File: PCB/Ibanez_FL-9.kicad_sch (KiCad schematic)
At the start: 156 parts, among them J1 INPUT, J2 OUTPUT, J3 EXT_DC, Q101 2SC2458GR, Q102 2SC2458GR, Q103 2SK44SPC, Q104 2SC2458GR, Q105 2SC2458GR, Q106 2SC2458GR, Q107 2SA1048Y/GR, Q108A1001 2SC1583F, Q108B1001 2SC1583F, Q109 2SC2458GR, SW1 NORMAL/EFFECT, U101 TL022, U102 TL022, U103 TL022, U104 MN3207, U105 MN3102, U106 LM78L05_TO92

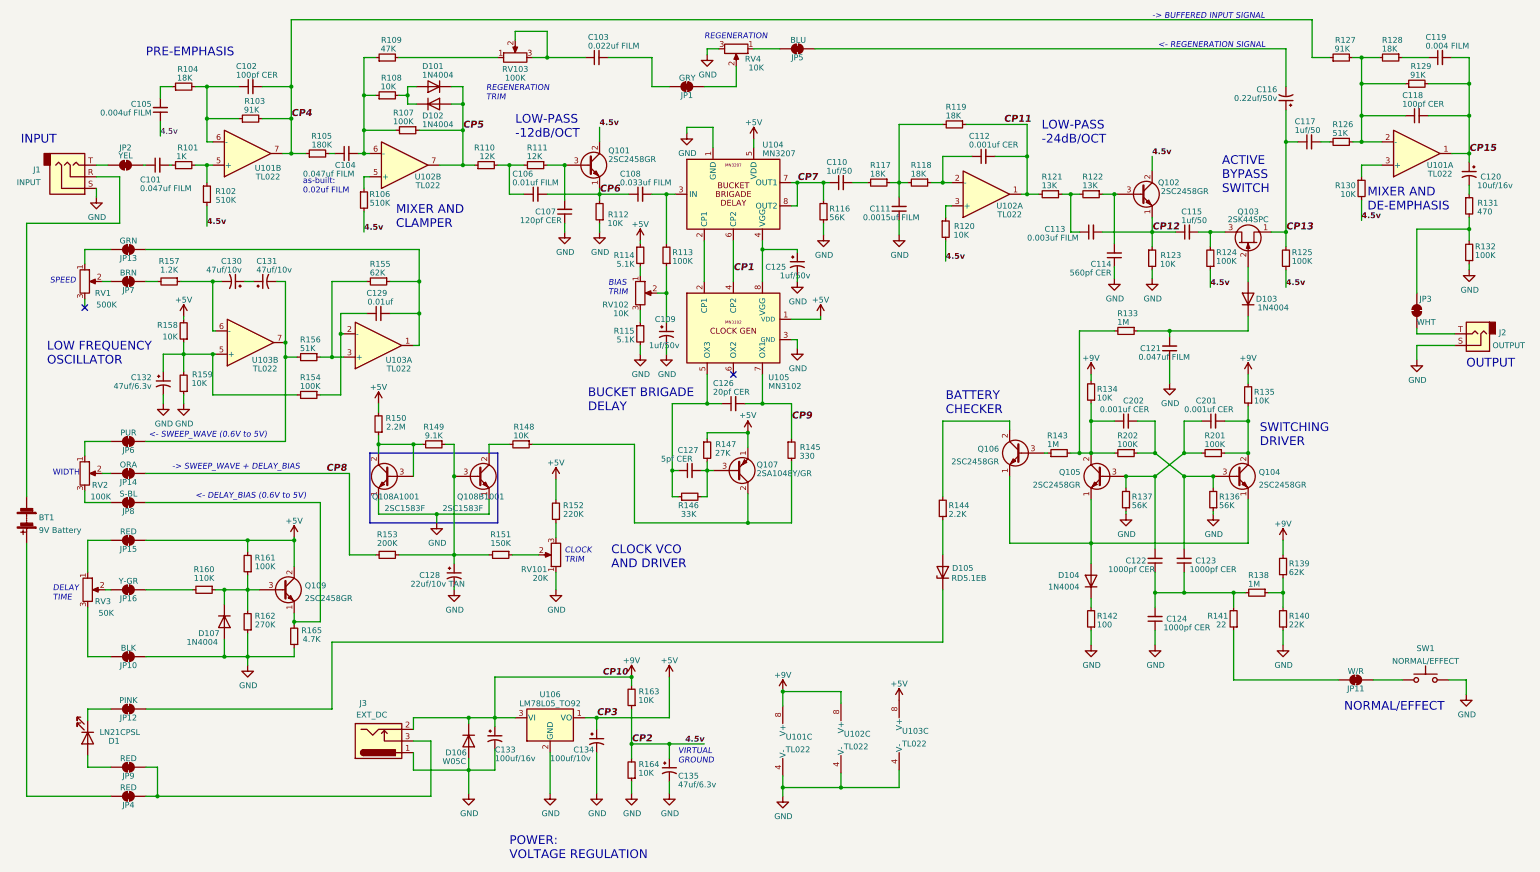
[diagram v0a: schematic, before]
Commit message: pcb layout v1.0
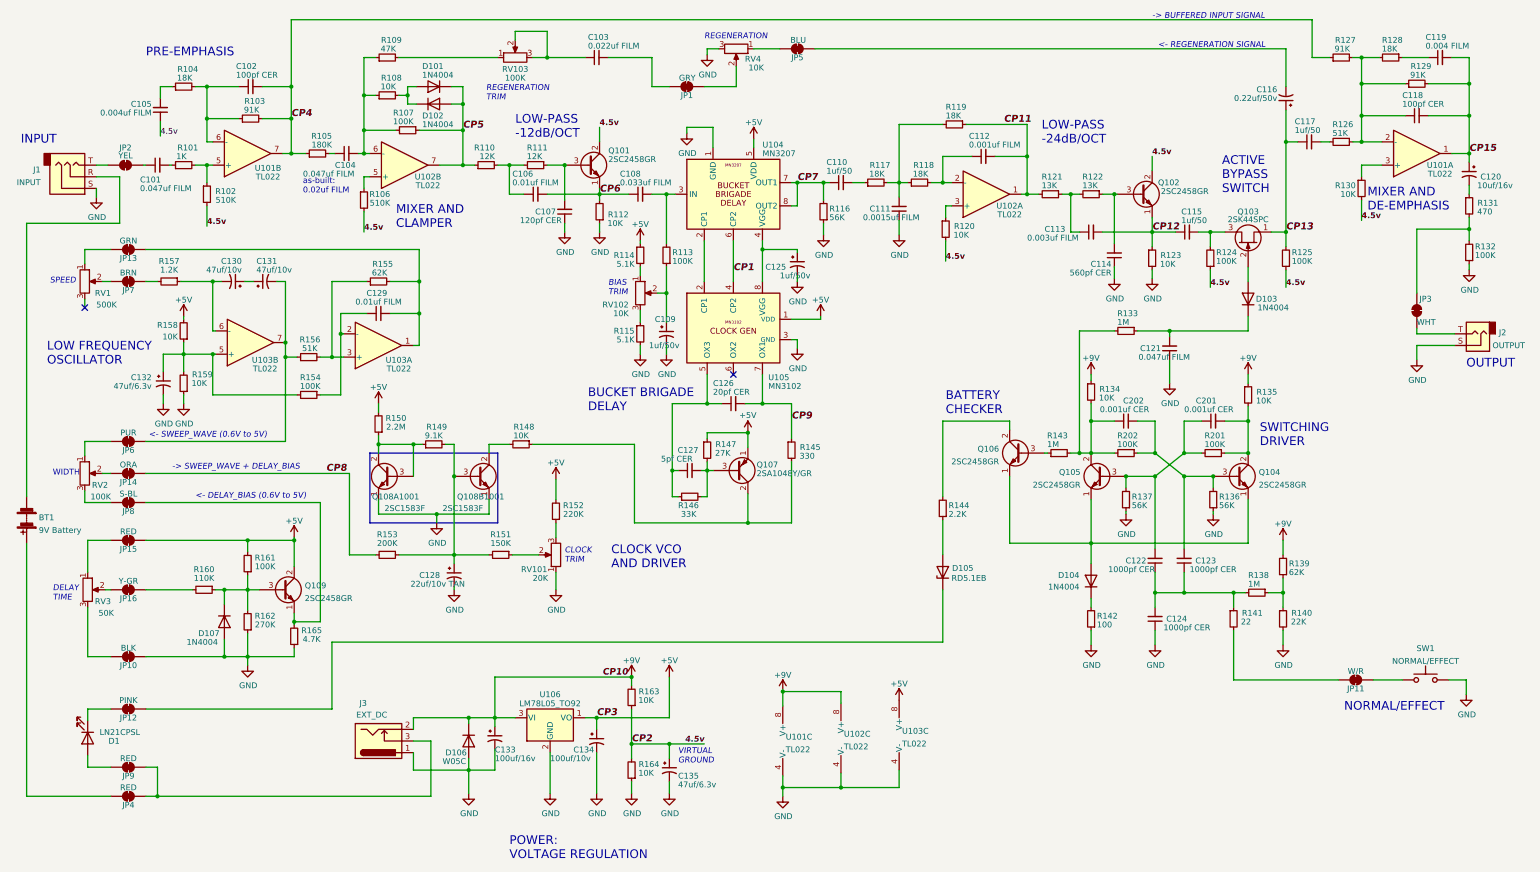
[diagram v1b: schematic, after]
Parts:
- BT1: footprint Battery:BatteryHolder_MPD_BA9VPC_1xPP3 -> (none)
- C111: footprint Capacitor_THT:C_Rect_L7.0mm_W2.5mm_P5.00mm -> Capacitor_THT:C_Rect_L7.0mm_W2.0mm_P5.00mm
- C112: value 0.001uf CER -> 0.001uf FILM; footprint Capacitor_THT:C_Disc_D3.0mm_W2.0mm_P2.50mm -> Capacitor_THT:C_Rect_L7.0mm_W2.0mm_P5.00mm
- C129: value 0.01uf -> 0.01uf FILM; footprint Capacitor_THT:C_Disc_D3.0mm_W2.0mm_P2.50mm -> Capacitor_THT:C_Rect_L7.0mm_W2.0mm_P5.00mm
- D1: footprint LED_THT:LED_D3.0mm_Clear -> (none)
- D105: footprint Diode_THT:D_DO-15_P2.54mm_Vertical_KathodeUp -> Diode_THT:D_T-1_P2.54mm_Vertical_KathodeUp
- RV1, RV2, RV3, RV4: footprint Potentiometer_THT:Potentiometer_ACP_CA6-H2,5_Horizontal -> (none)
- SW1: footprint Button_Switch_THT:SW_PUSH-12mm -> (none)
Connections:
- net +9V: now also R134.1, R135.1; no longer R134.2, R135.2
- net GND: now also R140.2; no longer R140.1
- net at C129.2, JP13.2 (B), U103.1: now also R155.2; no longer R155.1
- net at C202.1, Q105.2 (C), R133.2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: now also R134.2; no longer R134.1
- net at C110.2: now also R117.1; no longer R117.2
- net at C201.2, Q104.2 (C), R201.1: now also R135.2; no longer R135.1
- net at C122.1, C123.1, C124.2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: now also R141.1; no longer R141.2
- net at C112.1, U102.2 (-): now also R118.2; no longer R118.1
- net at C128.1, Q108B1001.3 (B), R151.2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: now also R149.2; no longer R149.1
- net at C111.2, R119.2: now also R117.2, R118.1; no longer R117.1, R118.2
- net at JP11.1 (A): now also R141.2; no longer R141.1
- net at Q108A1001.2 (C), Q108A1001.3 (B), R150.1: now also R149.1; no longer R149.2
- net at C131.2, JP6.2 (B), U103.7: now also R156.1; no longer R156.2
- net at R138.1, R139.1: now also R140.1; no longer R140.2
- new net: R155.1, R156.2, U103.3 (+)
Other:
- moved on the sheet: R117, R118, R134, R135, R140, R141, R149, R155, R156
